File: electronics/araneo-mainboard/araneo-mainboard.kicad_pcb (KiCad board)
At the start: 2 copper layers, 39 parts, among them J1 Conn_01x03_Pin, J10 Diode2, J11 Diode3, J12 OLED, J2 Conn_01x03_Pin, J3 Conn_01x03_Pin, J4 Conn_01x03_Pin, J5 Conn_01x03_Pin, J6 Conn_01x03_Pin, J7 Conn_01x03_Pin, J8 Conn_01x03_Pin, J9 Diode1, SW1 SW_SPST, U1 module_mpu6050, U2 L78M05CDT, U3 BD9C601EFJ

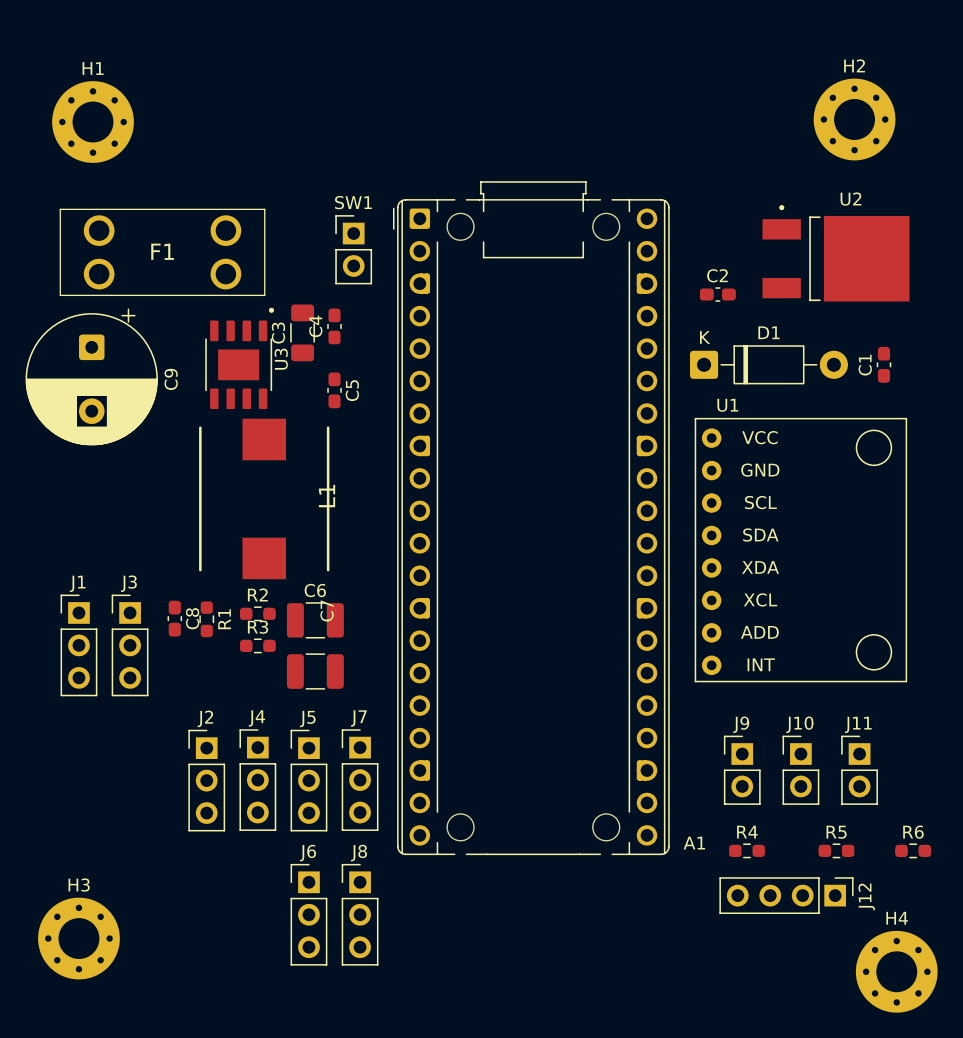
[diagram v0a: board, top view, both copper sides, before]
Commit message: electronics: full PCB
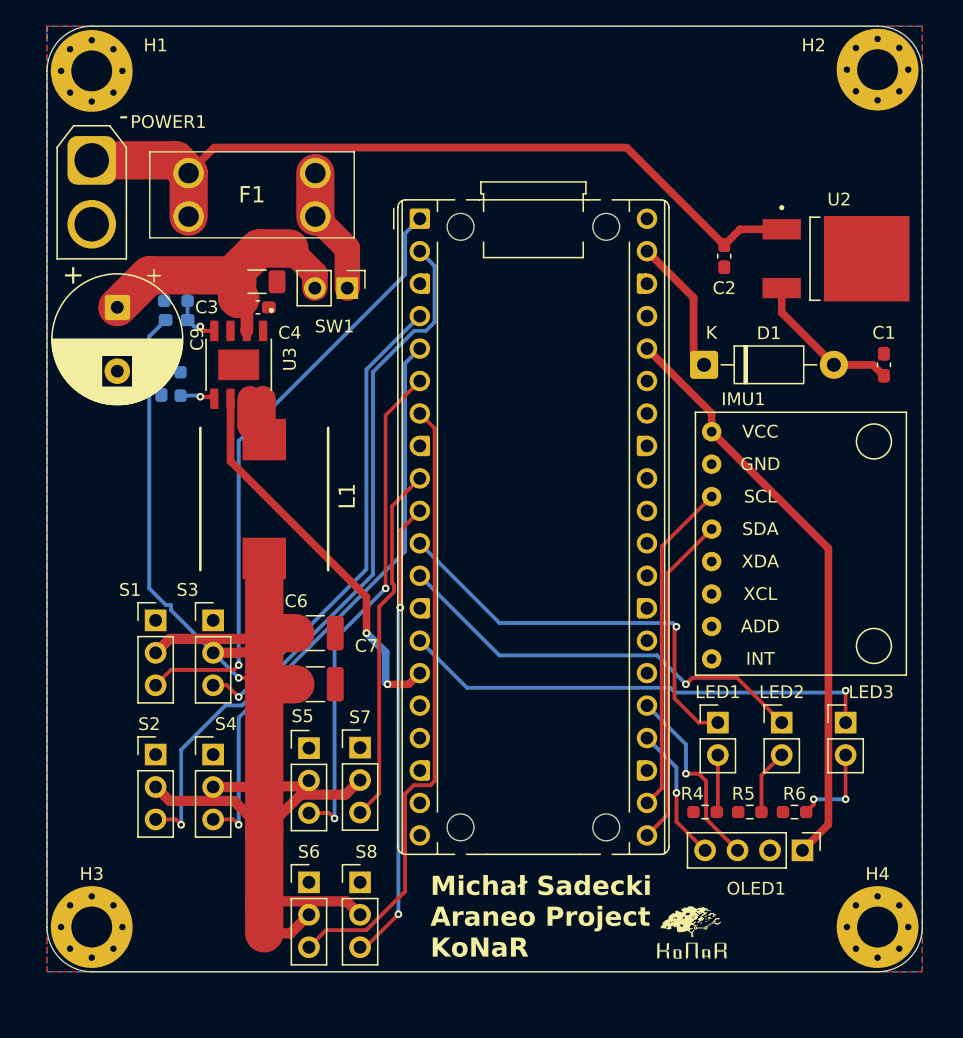
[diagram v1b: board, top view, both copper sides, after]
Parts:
- added ?: LOGO, Custom:konar, F.Cu at (145.0, 128.5)
- added POWER1: Conn_01x02_Pin, Connector_AMASS:AMASS_XT30U-M_1x02_P5.0mm_Vertical, F.Cu at (98.0, 68.0)
- C5: value C -> OPEN; moved to B.Cu
- C8: value C -> 1.5nF; moved to B.Cu
- R1: value R -> 1.2k; moved to B.Cu
- R2: value R -> 7.8k; moved to B.Cu
- R3: value R -> 39k; moved to B.Cu
- SW1: value SW_SPST -> SW
- moved R1 26.5 mm to (104.6, 77.5), turned to 0 degrees
- moved R2 25.3 mm to (104.6, 79.0), turned to 180 degrees
- moved R3 21.4 mm to (105.0, 85.5), turned to 90 degrees
- moved C8 18.4 mm to (103.5, 85.5)
- moved C5 13.5 mm to (104.6, 80.5), turned to 180 degrees
- moved R6 9.77 mm to (153.0, 119.0)
- moved F1 8.32 mm to (105.6, 72.4)
- moved R5 7.43 mm to (149.5, 119.0)
- moved S3 6.53 mm to (107.5, 104.0)
- moved C4 6.18 mm to (111.0, 79.5), turned to 180 degrees
- moved S1 6.03 mm to (103.0, 104.0)
- moved C3 5.36 mm to (110.9, 77.5), turned to 180 degrees
- moved R4 4.47 mm to (146.0, 119.0)
- moved OLED1 4.37 mm to (153.6, 122.0)
- moved SW1 4.30 mm to (118.0, 78.0), turned to -90 degrees
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- renumbered U1 to IMU1, J9 to LED1, J10 to LED2, J11 to LED3, J12 to OLED1, J1 to S1, J2 to S2, J3 to S3, J4 to S4, J5 to S5, J6 to S6, J7 to S7, J8 to S8
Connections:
- C8 pad 1: Net-(U3-COMP) -> Net-(C8-Pad1)
- C8 pad 2: Net-(C8-Pad2) -> GND
- R3 pad 1: Net-(C8-Pad2) -> Net-(U3-COMP)
- R3 pad 2: GND -> Net-(C8-Pad1)
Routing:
- net +6V: track 0.00 -> 120.2 mm, vias 0 -> 1
- net +7.4V: track 0.00 -> 62.3 mm
- net PWM2: track 0.00 -> 57.1 mm, vias 0 -> 1
- net PWM6: track 0.00 -> 48.9 mm
- net PWM1: track 0.00 -> 48.0 mm, vias 0 -> 1
- net +3V3: track 0.00 -> 46.0 mm
- net PWM4: track 0.00 -> 45.3 mm, vias 0 -> 1
- net PWM5: track 0.00 -> 39.2 mm, vias 0 -> 2
- net PWM3: track 0.00 -> 38.1 mm, vias 0 -> 1
- net D3: track 0.00 -> 37.6 mm, vias 0 -> 1
- net PWM8: track 0.00 -> 36.4 mm, vias 0 -> 2
- net D2: track 0.00 -> 33.5 mm, vias 0 -> 1
- net D1: track 0.00 -> 32.6 mm, vias 0 -> 1
- net EN: track 0.00 -> 30.3 mm, vias 0 -> 2
- net PWM7: track 0.00 -> 28.2 mm
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- added copper zone on B.Cu, net GND
- added copper zone on F.Cu, net GND
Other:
- board outline added: 68.5 x 74 mm
- board text added: "15.07.2026 Projekt inżynierski prowadzony przez Mateusza Cholewińskiego"
- board text added: "Michał Sadecki Araneo Project KoNaR"
